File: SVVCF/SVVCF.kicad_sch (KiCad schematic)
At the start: 58 parts, among them J1 Conn_02x05_Top_Bottom, J2 Conn_01x14_Pin, Q1 2N3904, U1 TL072, U2 TL072, U3 PT2399, U4 LM7805_TO220

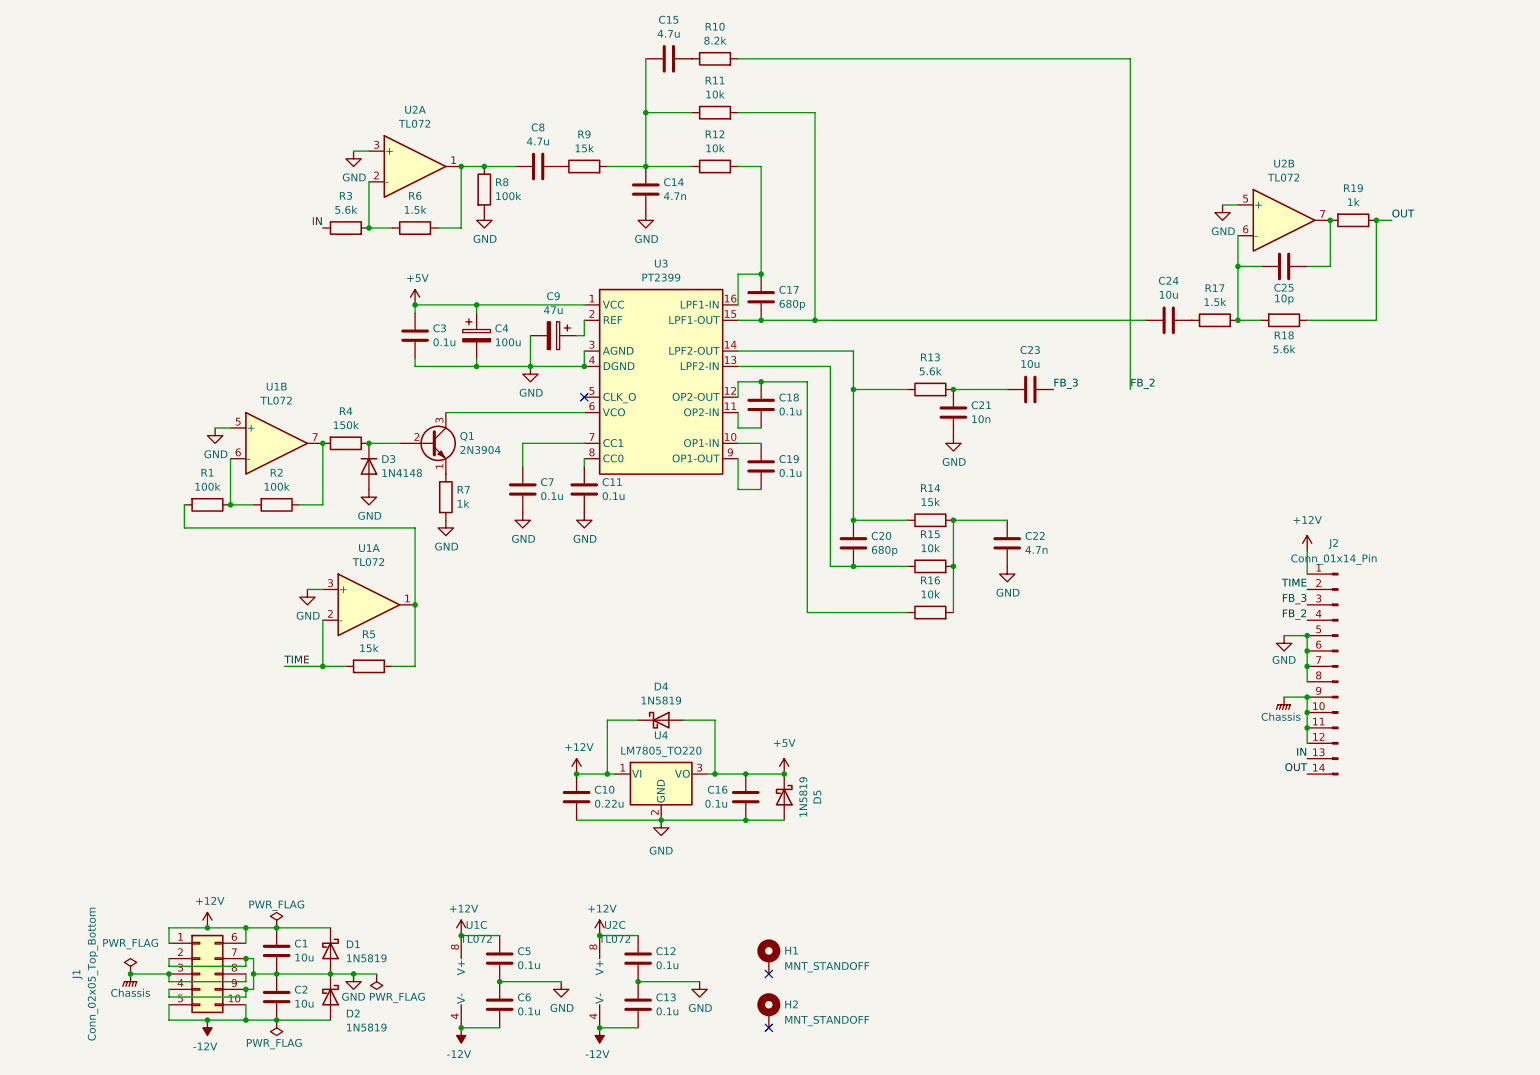
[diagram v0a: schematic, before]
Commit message: Begin revised delay
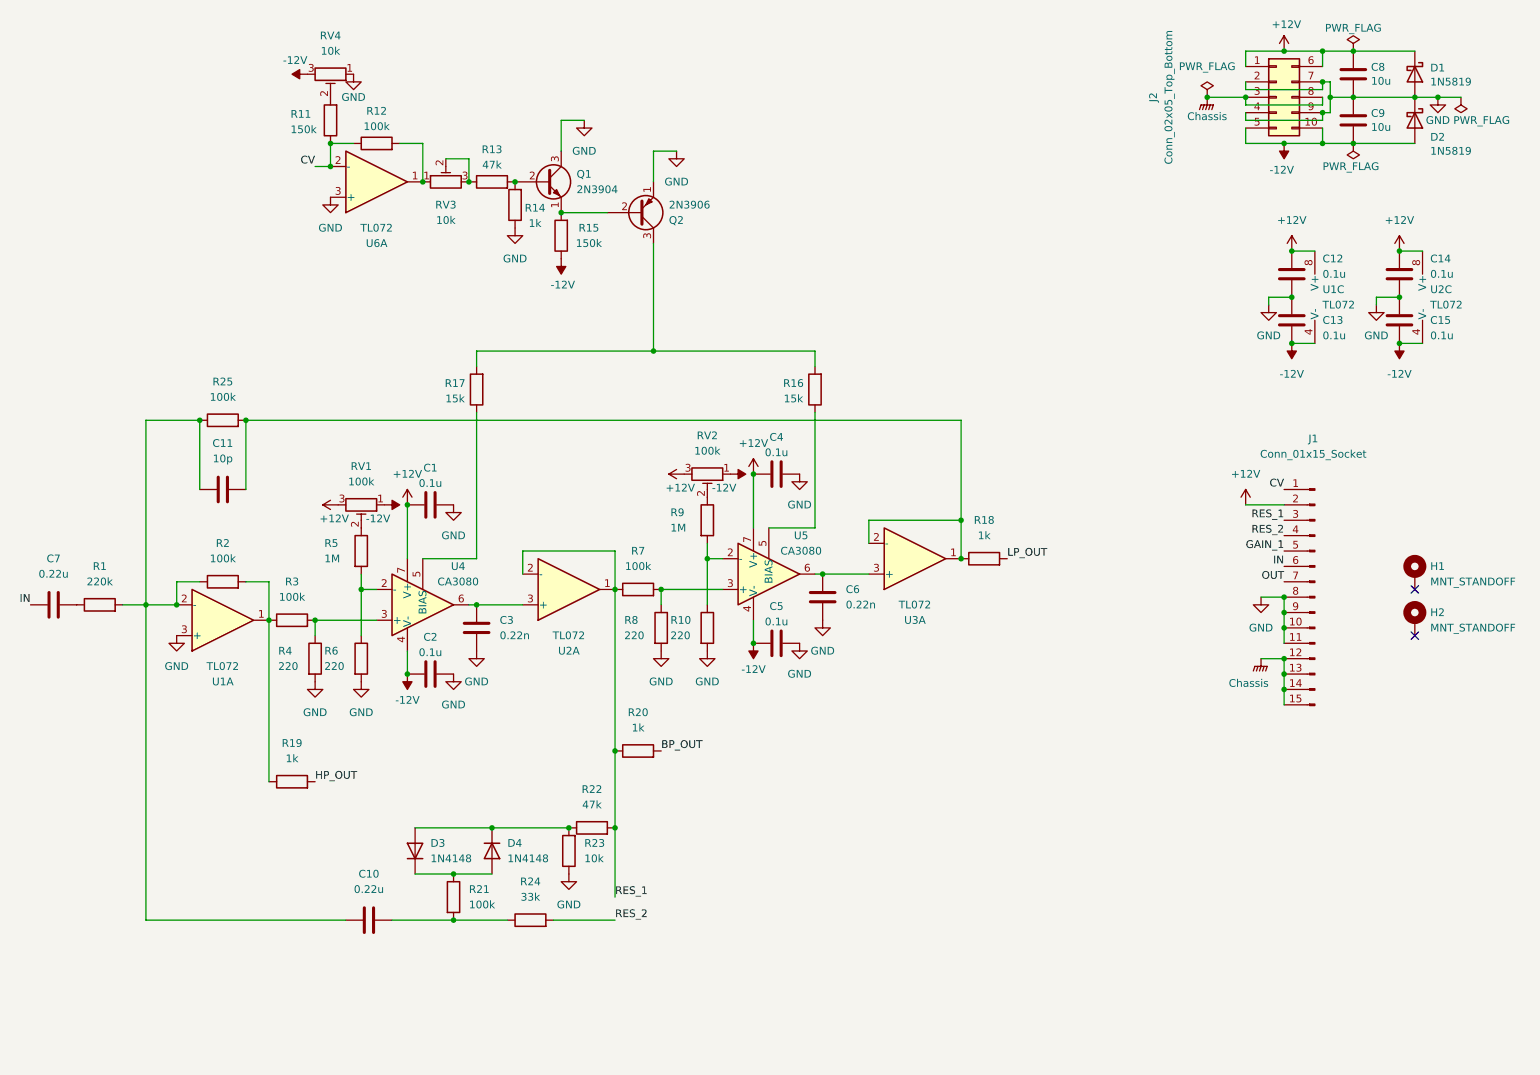
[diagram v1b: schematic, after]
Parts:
- removed C16, C18, C19: 0.1u, 0_Capacitor_THT:C_Disc_D5.5mm_W2.5mm_P2.50mm, symbol Device:C
- removed C17, C20: 680p, 0_Capacitor_THT:C_Disc_D5.5mm_W2.5mm_P2.50mm, symbol Device:C
- removed C21: 10n, 0_Capacitor_THT:C_Disc_D5.5mm_W2.5mm_P2.50mm, symbol Device:C
- removed C22: 4.7n, 0_Capacitor_THT:C_Disc_D5.5mm_W2.5mm_P2.50mm, symbol Device:C
- removed C23, C24: 10u, 0_Capacitor_THT:C_Disc_D5.5mm_W4.0mm_P2.50mm, symbol Device:C
- removed C25: 10p, 0_Capacitor_THT:C_Disc_D5.5mm_W2.5mm_P2.50mm, symbol Device:C
- removed C4: 100u, Capacitor_THT:CP_Radial_D6.3mm_P2.50mm, symbol Device:C_Polarized
- removed C9: 47u, Capacitor_THT:CP_Radial_D5.0mm_P2.50mm, symbol Device:C_Polarized
- removed D4, D5: 1N5819, Diode_THT:D_DO-41_SOD81_P10.16mm_Horizontal, symbol Diode:1N5819
- removed J1: Conn_02x05_Top_Bottom, Connector_Molex:Molex_Mini-Fit_Jr_5566-10A_2x05_P4.20mm_Vertical, symbol Connector_Generic:Conn_02x05_Top_Bottom
- removed J2: Conn_01x14_Pin, Connector_PinHeader_2.54mm:PinHeader_1x14_P2.54mm_Vertical, symbol Connector:Conn_01x14_Pin
- removed unit 2 of U1
- removed unit 2 of U2
- removed U3: PT2399, Package_DIP:DIP-16_W7.62mm, symbol Audio:PT2399
- removed U4: LM7805_TO220, Package_TO_SOT_THT:TO-220-3_Vertical, symbol Regulator_Linear:LM7805_TO220
- added C4: 0.1u, symbol Device:C
- added C9: 10u, 0_Capacitor_THT:C_Disc_D5.5mm_W4.0mm_P2.50mm, symbol Device:C
- added D4: 1N4148, Diode_THT:D_DO-35_SOD27_P7.62mm_Horizontal, symbol Diode:1N4148
- added J1: Conn_01x15_Socket, Connector_PinHeader_2.54mm:PinHeader_1x15_P2.54mm_Vertical, symbol Connector:Conn_01x15_Pin
- added J2: Conn_02x05_Top_Bottom, Connector_Molex:Molex_Mini-Fit_Jr_5566-10A_2x05_P4.20mm_Vertical, symbol Connector_Generic:Conn_02x05_Top_Bottom
- added Q2: 2N3906, Package_TO_SOT_THT:TO-92_Inline, symbol Transistor_BJT:2N3906
- added R20: 1k, symbol Device:R
- added R21, R25: 100k, symbol Device:R
- added R22: 47k, symbol Device:R
- added R23: 10k, symbol Device:R
- added R24: 33k, symbol Device:R
- added RV1, RV2: 100k, symbol Device:R_Potentiometer_Trim
- added RV3, RV4: 10k, symbol Device:R_Potentiometer_Trim
- added U3, U6: TL072, symbol Amplifier_Operational:TL072
- added U4, U5: CA3080, symbol Amplifier_Operational:CA3080
- C1, C2: value 10u -> 0.1u; footprint 0_Capacitor_THT:C_Disc_D5.5mm_W4.0mm_P2.50mm -> (none)
- C10, C5: footprint 0_Capacitor_THT:C_Disc_D5.5mm_W2.5mm_P2.50mm -> (none)
- C11: value 0.1u -> 10p; footprint 0_Capacitor_THT:C_Disc_D5.5mm_W2.5mm_P2.50mm -> (none)
- C14: value 4.7n -> 0.1u
- C15: value 4.7u -> 0.1u; footprint Capacitor_THT:C_Disc_D3.8mm_W2.6mm_P2.50mm -> 0_Capacitor_THT:C_Disc_D5.5mm_W2.5mm_P2.50mm
- C3, C6: value 0.1u -> 0.22n; footprint 0_Capacitor_THT:C_Disc_D5.5mm_W2.5mm_P2.50mm -> (none)
- C7: value 0.1u -> 0.22u; footprint 0_Capacitor_THT:C_Disc_D5.5mm_W2.5mm_P2.50mm -> (none)
- C8: value 4.7u -> 10u; footprint Capacitor_THT:C_Disc_D3.8mm_W2.6mm_P2.50mm -> 0_Capacitor_THT:C_Disc_D5.5mm_W4.0mm_P2.50mm
- Q1: footprint Package_TO_SOT_THT:TO-92_HandSolder -> Package_TO_SOT_THT:TO-92_Inline
- R1: value 100k -> 220k; footprint Resistor_THT:R_Axial_DIN0207_L6.3mm_D2.5mm_P7.62mm_Horizontal -> (none)
- R10: value 8.2k -> 220; footprint Resistor_THT:R_Axial_DIN0207_L6.3mm_D2.5mm_P7.62mm_Horizontal -> (none)
- R11, R15: value 10k -> 150k; footprint Resistor_THT:R_Axial_DIN0207_L6.3mm_D2.5mm_P7.62mm_Horizontal -> (none)
- R12: value 10k -> 100k; footprint Resistor_THT:R_Axial_DIN0207_L6.3mm_D2.5mm_P7.62mm_Horizontal -> (none)
- R13: value 5.6k -> 47k; footprint Resistor_THT:R_Axial_DIN0207_L6.3mm_D2.5mm_P7.62mm_Horizontal -> (none)
- R14: value 15k -> 1k; footprint Resistor_THT:R_Axial_DIN0207_L6.3mm_D2.5mm_P7.62mm_Horizontal -> (none)
- R16: value 10k -> 15k; footprint Resistor_THT:R_Axial_DIN0207_L6.3mm_D2.5mm_P7.62mm_Horizontal -> (none)
- R17: value 1.5k -> 15k; footprint Resistor_THT:R_Axial_DIN0207_L6.3mm_D2.5mm_P7.62mm_Horizontal -> (none)
- R18: value 5.6k -> 1k; footprint Resistor_THT:R_Axial_DIN0207_L6.3mm_D2.5mm_P7.62mm_Horizontal -> (none)
- R19, R2: footprint Resistor_THT:R_Axial_DIN0207_L6.3mm_D2.5mm_P7.62mm_Horizontal -> (none)
- R3: value 5.6k -> 100k; footprint Resistor_THT:R_Axial_DIN0207_L6.3mm_D2.5mm_P7.62mm_Horizontal -> (none)
- R4: value 150k -> 220; footprint Resistor_THT:R_Axial_DIN0207_L6.3mm_D2.5mm_P7.62mm_Horizontal -> (none)
- R5, R9: value 15k -> 1M; footprint Resistor_THT:R_Axial_DIN0207_L6.3mm_D2.5mm_P7.62mm_Horizontal -> (none)
- R6: value 1.5k -> 220; footprint Resistor_THT:R_Axial_DIN0207_L6.3mm_D2.5mm_P7.62mm_Horizontal -> (none)
- R7: value 1k -> 100k; footprint Resistor_THT:R_Axial_DIN0207_L6.3mm_D2.5mm_P7.62mm_Horizontal -> (none)
- R8: value 100k -> 220; footprint Resistor_THT:R_Axial_DIN0207_L6.3mm_D2.5mm_P7.62mm_Horizontal -> (none)
- U1, U2: footprint Package_DIP:DIP-8_W7.62mm_Socket -> (none)
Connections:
- net FB_2 is gone; now on net GND: R10.2
- net +12V: now also C12.2, C14.2, C8.1, C4.1, J1.2 (Pin_2), J2.1 (Pin_1), J2.6 (Pin_6), RV1.3, RV2.3, U4.7 (V+), U5.7 (V+); no longer C10.1, C12.1, C5.1
- net -12V: now also C13.1, C15.1, C2.1, C5.1, R15.1, C9.2, J2.10 (Pin_10), J2.5 (Pin_5), RV1.1, RV2.1, RV4.3, U4.4 (V-), U5.4 (V-); no longer C13.2, C2.2, C6.2
- net Chassis: now also J1.12 (Pin_12), J1.13 (Pin_13), J1.14 (Pin_14), J1.15 (Pin_15), J2.3 (Pin_3), J2.8 (Pin_8)
- net GND: now also C12.1, C13.2, C14.1, C15.2, C2.2, C6.2, C8.2, Q1.3 (C), R14.1, R4.2, R6.2, C4.2, C9.1, J1.10 (Pin_10), J1.11 (Pin_11), J1.8 (Pin_8), J1.9 (Pin_9), J2.2 (Pin_2), J2.4 (Pin_4), J2.7 (Pin_7), J2.9 (Pin_9), Q2.1 (E), R23.1, RV4.1, U6.3 (+); no longer C10.2, C11.2, C12.2, C13.1, C14.2, C2.1, C6.1, C7.2, D3.2 (A), R7.2, U2.3 (+)
- net IN: now also C7.1, J1.6 (Pin_6); no longer R3.1
- net OUT: now also J1.7 (Pin_7); no longer R18.1, R19.1
- net at R1.1: now also C7.2; no longer R2.2
- net at R2.1: now also C10.1, C11.1, R1.2, U1.2 (-), R25.1; no longer R4.2
- net at R16.1: now also U5.5 (BIAS)
- net at R13.1: now also RV3.2, RV3.3; no longer R14.1
- net at R11.2: now also RV4.2
- net at R12.2: now also RV3.1, U6.1
- net at R10.1: now also R9.2, U5.2 (-); no longer C15.1
- net at R13.2: now also Q1.2 (B), R14.2
- net at R9.1: now also RV2.2; no longer C8.1
- net at R17.2: now also R16.2, Q2.3 (C); no longer R18.2
- net HP_OUT: now reaches R19.2
- net at R17.1: now also U4.5 (BIAS)
- net at Q1.1 (E): now also R15.2, Q2.2 (B); no longer R7.1
- net +5V: no longer names the net of C3.1
- net +5V: now also U2.3 (+), U4.6
- net TIME: no longer names the net of R5.2
- net TIME: now also R6.1, U4.2 (-); no longer U1.2 (-)
- new net: D3.2 (A), D4.1 (K), R22.1, R23.2
- new net: D3.1 (K), D4.2 (A), R21.1
- new net: R5.1, RV1.2
- new net: R7.2, R8.1, U5.3 (+)
- new net: C11.2, R18.1, R25.2, U3.1, U3.2 (-)
- new net: C6.1, U3.3 (+), U5.6
- new net: C10.2, R21.2, R24.1
- new net: R19.1, R2.2, R3.1, U1.1
- new net: R3.2, R4.1, U4.3 (+)
- new net BP_OUT: R20.2
- new net CV: J1.1 (Pin_1), R11.1, R12.1, U6.2 (-)
- new net GAIN_1: J1.5 (Pin_5)
- new net LP_OUT: R18.2
- new net RES_1: J1.3 (Pin_3), R20.1, R22.2, R7.1, U2.1, U2.2 (-)
- new net RES_2: J1.4 (Pin_4), R24.2
- no-connect marks 3 -> 2
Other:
- title: Delay -> (none)
